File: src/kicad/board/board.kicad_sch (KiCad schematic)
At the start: 19 parts, among them U1 Pico

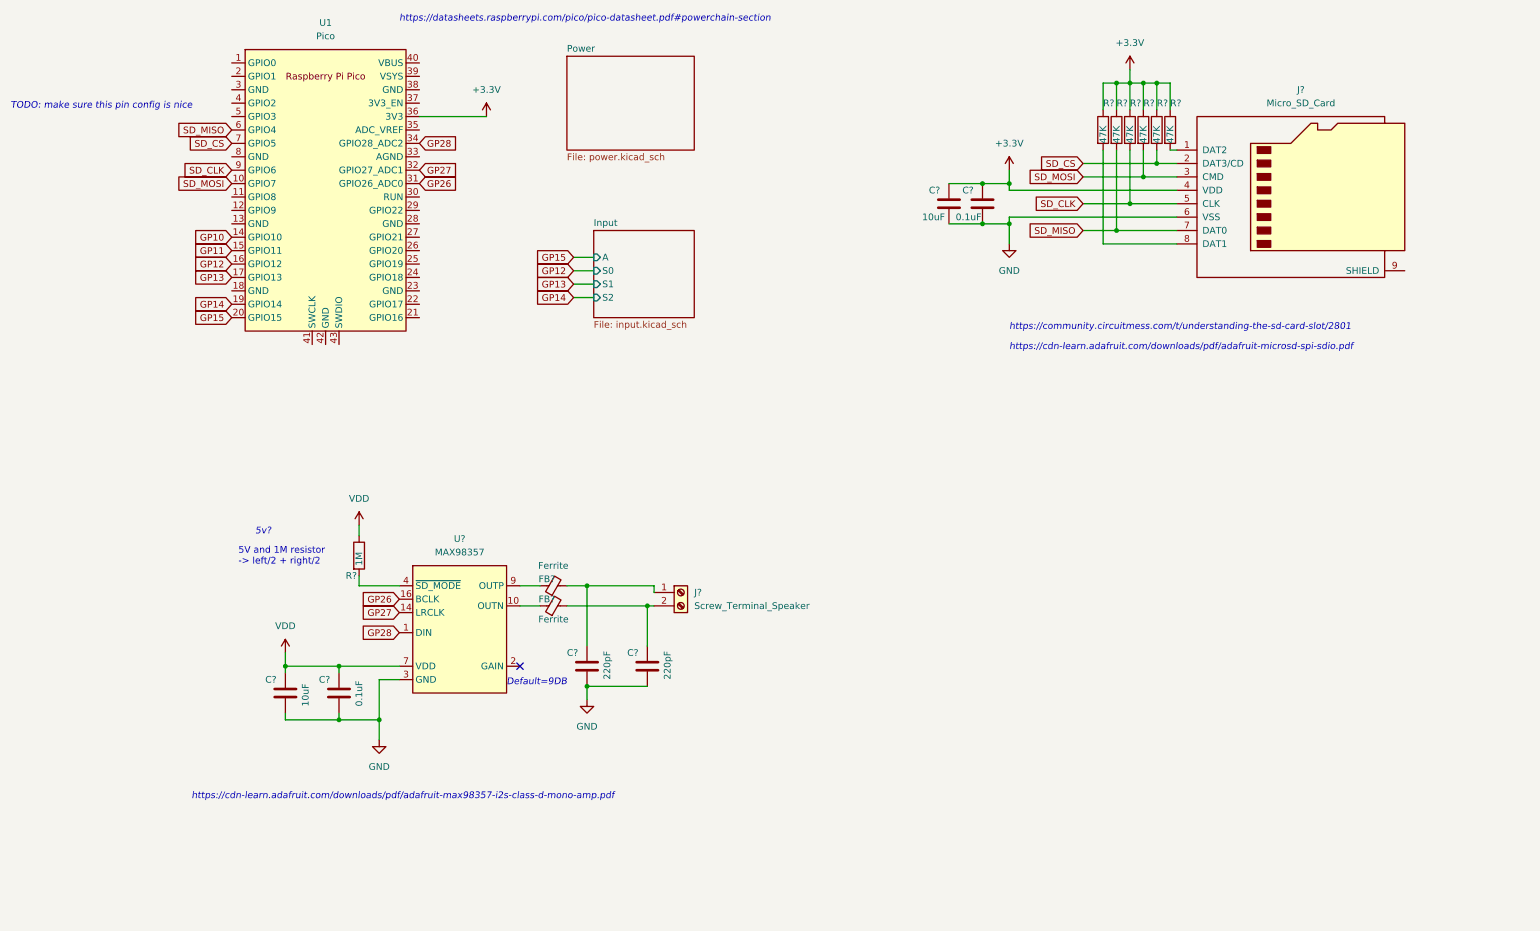
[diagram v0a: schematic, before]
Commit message: update pcb
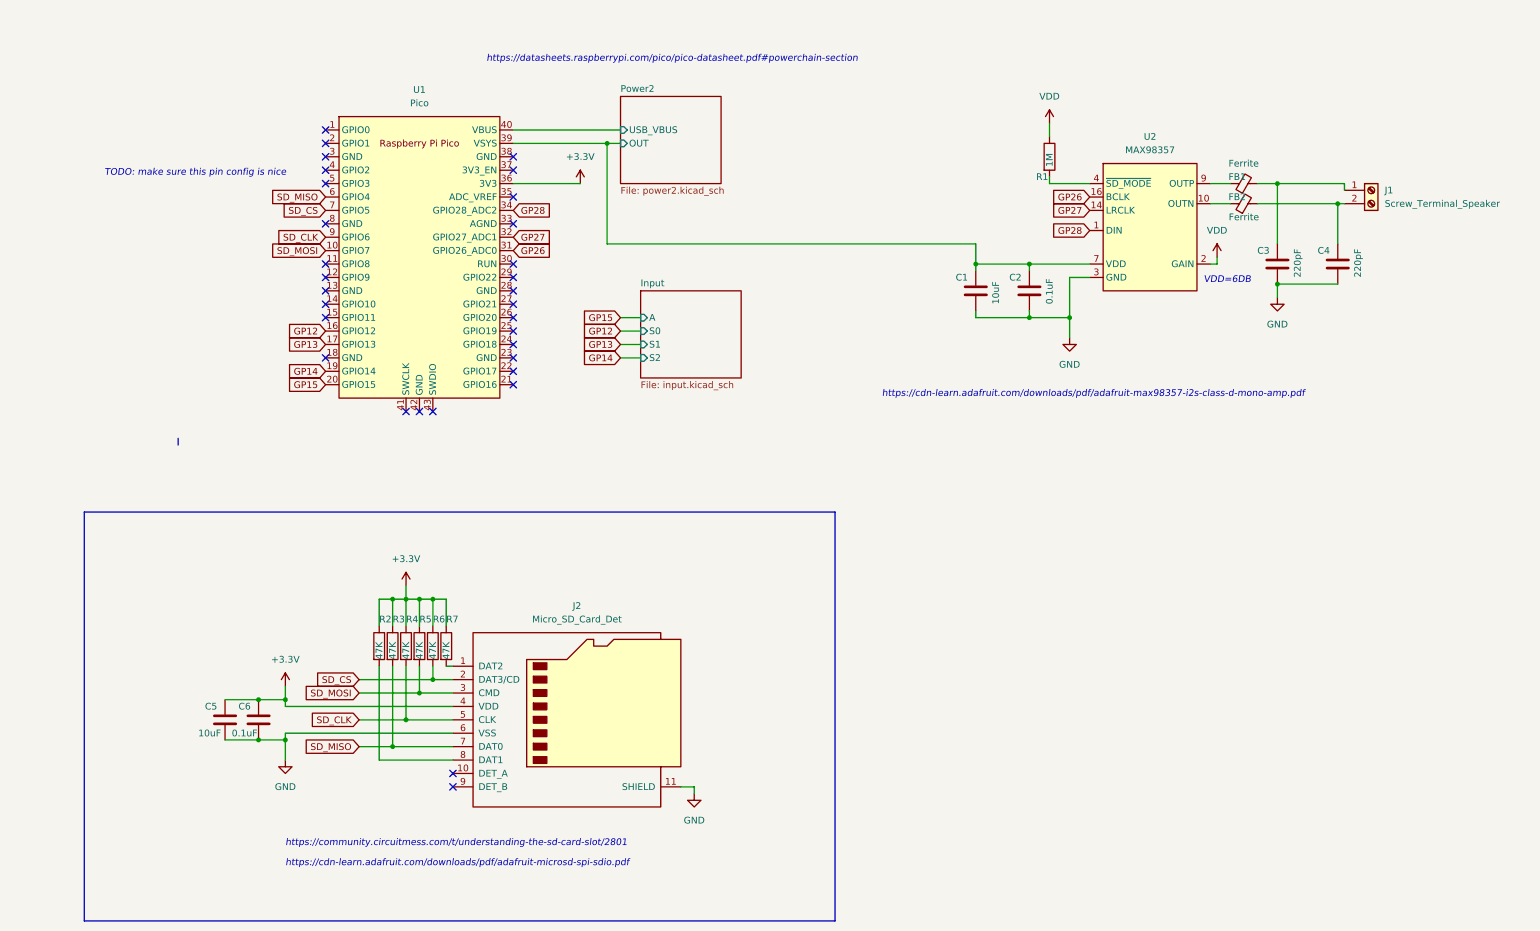
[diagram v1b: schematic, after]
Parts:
- removed J?: Micro_SD_Card, symbol Connector:Micro_SD_Card
- added J2: Micro_SD_Card_Det, Connector_Card:microSD_HC_Molex_104031-0811, symbol Connector:Micro_SD_Card_Det
- C1, C2, C3, C4, C5, C6: renamed from C?; footprint (none) -> Capacitor_SMD:C_0805_2012Metric
- R1, R2, R3, R4, R5, R6, R7: renamed from R?; footprint (none) -> Resistor_SMD:R_0805_2012Metric
- U2: renamed from U?; footprint (none) -> Library:MAX98357
- gave numbers to parts that had none: 3
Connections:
- net +3.3V: now also J2.4 (VDD)
- net GND: now also J2.11 (SHIELD), J2.6 (VSS)
- net SD_CLK: now also J2.5 (CLK)
- net SD_CS: now also J2.2 (DAT3/CD)
- net SD_MISO: now also J2.7 (DAT0)
- net SD_MOSI: now also J2.3 (CMD)
- net VDD: now also U1.39 (VSYS), U2.2 (GAIN)
- net at R7.2: now also J2.1 (DAT2)
- net Power2/USB_VBUS: now reaches U1.40 (VBUS)
- net at R2.2: now also J2.8 (DAT1)
- net GP10: no longer names the net of U1.14 (GPIO10)
- net GP11: no longer names the net of U1.15 (GPIO11)
- no-connect marks 1 -> 31
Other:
- removed sheet Power
- added sheet Power2 (power2.kicad_sch)
- note added: "VDD=6DB"
- note removed: "5V and 1M resistor -> left/2 + right/2"
- note removed: "5v?"
- note removed: "Default=9DB"
- moved on the sheet: C1, C2, C3, C4, C5, C6, FB1, FB2, J1, R1, R2, R3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
